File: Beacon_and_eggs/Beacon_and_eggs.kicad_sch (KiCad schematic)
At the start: 41 parts, among them J1 USB_C_Receptacle_USB2.0_16P, Q1 IRLML0030, SW1 Boot, SW2 Reset, U1 SA818V, U2 STM32F411CEUx, U3 ADXL343, U6 MCP1253-33X50I/MS, U7 MCP1253-33X50I/MS, Y1 25MHz 18pF, Y2 32.768kHz 12.5pF

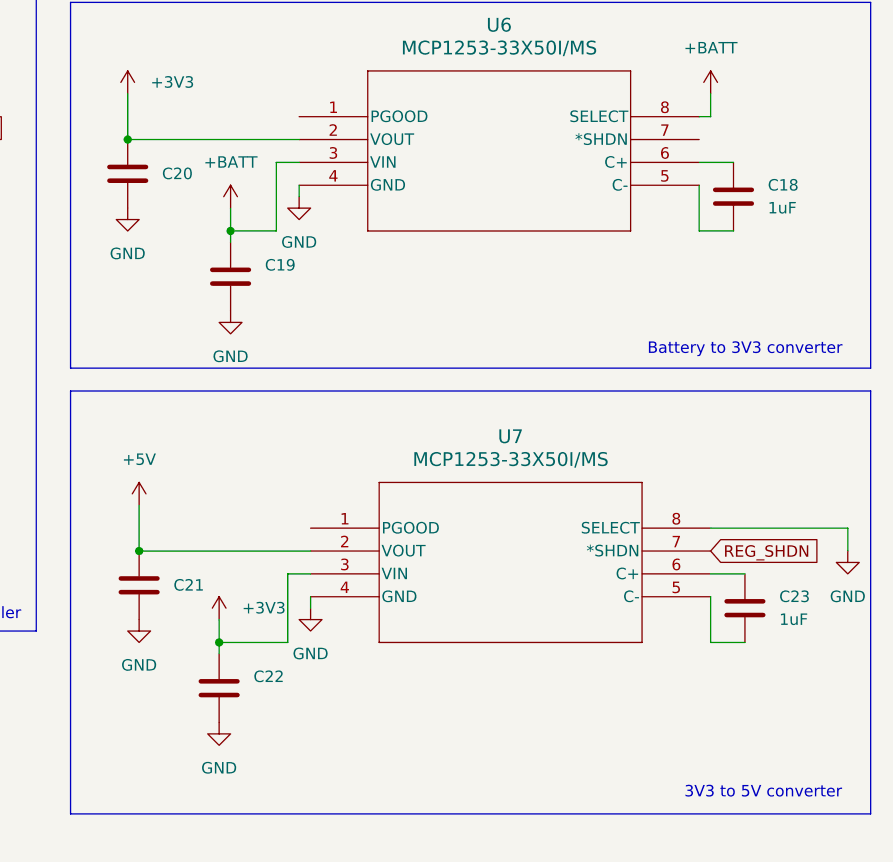
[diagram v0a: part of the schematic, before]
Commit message: Assingned most components(1206 for resistors and Capacitors)
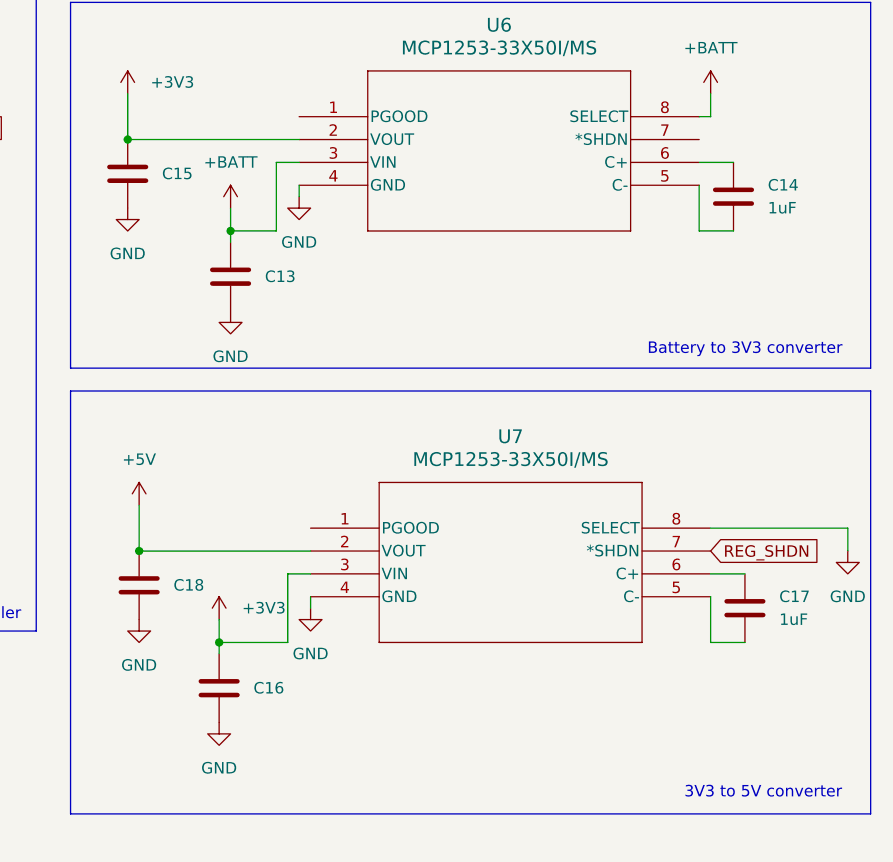
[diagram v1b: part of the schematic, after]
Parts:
- BZ1: footprint (none) -> Buzzer_Beeper:MagneticBuzzer_PUI_SMT-1028-T-2-R
- C1, C10, C11, C12, C2, C3, C4, C5, C6, C7, C8, C9: footprint (none) -> Capacitor_SMD:C_1206_3216Metric
- J1: footprint (none) -> Connector_USB:USB_C_Receptacle_HCTL_HC-TYPE-C-16P-01A
- R1, R2, R3, R4, R5, R6, R7, R8, R9: footprint (none) -> Resistor_SMD:R_1206_3216Metric
- SW1, SW2: footprint (none) -> Button_Switch_SMD:SW_SPST_PTS810
- U6, U7: footprint MSOP8_MC_MCH -> 2025_26-UVR-Beacon:MSOP8_MC_MCH
- renumbered C19 to C13, C18 to C14, C20 to C15, C22 to C16, C23 to C17, C21 to C18
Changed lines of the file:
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@@
 			)
 		)
-		(property "Footprint" ""
+		(property "Footprint" "Capacitor_SMD:C_1206_3216Metric"
 			(at 109.22 119.6848 0)
 			(effects
@@
 			)
 		)
-		(property "Footprint" "MSOP8_MC_MCH"
+		(property "Footprint" "2025_26-UVR-Beacon:MSOP8_MC_MCH"
 			(at 212.598 118.872 0)
 			(effects
@@
 			)
 		)
-		(property "Footprint" ""
+		(property "Footprint" "Resistor_SMD:R_1206_3216Metric"
 			(at 28.448 80.01 90)
 			(effects
@@
 			)
 		)
-		(property "Footprint" ""
+		(property "Footprint" "Connector_USB:USB_C_Receptacle_HCTL_HC-TYPE-C-16P-01A"
 			(at 34.29 134.62 0)
 			(effects
@@
 			)
 		)
-		(property "Footprint" ""
+		(property "Footprint" "Resistor_SMD:R_1206_3216Metric"
 			(at 31.75 41.148 90)
 			(effects
@@
 			)
 		)
-		(property "Footprint" ""
+		(property "Footprint" "Capacitor_SMD:C_1206_3216Metric"
 			(at 148.59 34.5948 0)
 			(effects
@@
 			)
 		)
-		(property "Footprint" ""
+		(property "Footprint" "Resistor_SMD:R_1206_3216Metric"
 			(at 52.07 130.048 90)
 			(effects
@@
 			)
 		)
-		(property "Footprint" ""
+		(property "Footprint" "Capacitor_SMD:C_1206_3216Metric"
 			(at 40.64 65.0748 0)
 			(effects
@@
 		(dnp no)
 		(fields_autoplaced yes)
-		(property "Reference" "C19"
-			(at 215.9 100.3299 0)
+		(property "Reference" "C13"
+			(at 215.9 101.5999 0)
 			(effects
 				(font
@@
 			(project "Beacon_and_eggs"
 				(path "/8792c0a0-2ad2-47f4-a55d-c9a646f00347"
-					(reference "C19")
+					(reference "C13")
 					(unit 1)
 				)
@@
 			)
 		)
-		(property "Footprint" ""
+		(property "Footprint" "Resistor_SMD:R_1206_3216Metric"
 			(at 24.638 80.01 90)
 			(effects
@@
 		(dnp no)
 		(fields_autoplaced yes)
-		(property "Reference" "C20"
+		(property "Reference" "C15"
 			(at 204.47 90.1699 0)
 			(effects
@@
 			(project "Beacon_and_eggs"
 				(path "/8792c0a0-2ad2-47f4-a55d-c9a646f00347"
-					(reference "C20")
+					(reference "C15")
 					(unit 1)
 				)
@@
 			)
 		)
-		(property "Footprint" ""
+		(property "Footprint" "Capacitor_SMD:C_1206_3216Metric"
 			(at 161.29 34.5948 0)
 			(effects
@@
 		(dnp no)
 		(fields_autoplaced yes)
-		(property "Reference" "C22"
-			(at 214.63 146.0499 0)
+		(property "Reference" "C16"
+			(at 214.63 147.3199 0)
 			(effects
 				(font
@@
 			(project "Beacon_and_eggs"
 				(path "/8792c0a0-2ad2-47f4-a55d-c9a646f00347"
-					(reference "C22")
+					(reference "C16")
 					(unit 1)
 				)
@@
 			)
 		)
-		(property "Footprint" ""
+		(property "Footprint" "Capacitor_SMD:C_1206_3216Metric"
 			(at 35.56 47.2948 0)
 			(effects
@@
 		(dnp no)
 		(fields_autoplaced yes)
-		(property "Reference" "C21"
+		(property "Reference" "C18"
 			(at 205.74 135.8899 0)
 			(effects
@@
 			(project "Beacon_and_eggs"
 				(path "/8792c0a0-2ad2-47f4-a55d-c9a646f00347"
-					(reference "C21")
+					(reference "C18")
 					(unit 1)
 				)
@@
 			)
 		)
-		(property "Footprint" ""
+		(property "Footprint" "Resistor_SMD:R_1206_3216Metric"
 			(at 64.008 30.48 90)
 			(effects
@@
 			)
 		)
-		(property "Footprint" ""
+		(property "Footprint" "Capacitor_SMD:C_1206_3216Metric"
 			(at 148.59 23.1648 0)
 			(effects
@@
 			)
 		)
-		(property "Footprint" ""
+		(property "Footprint" "Resistor_SMD:R_1206_3216Metric"
 			(at 108.712 170.18 90)
 			(effects
@@
 		(dnp no)
 		(fields_autoplaced yes)
-		(property "Reference" "C23"
+		(property "Reference" "C17"
 			(at 273.05 137.1599 0)
 			(effects
@@
 			(project "Beacon_and_eggs"
 				(path "/8792c0a0-2ad2-47f4-a55d-c9a646f00347"
-					(reference "C23")
+					(reference "C17")
 					(unit 1)
 				)
@@
 			)
 		)
-		(property "Footprint" ""
+		(property "Footprint" "Resistor_SMD:R_1206_3216Metric"
 			(at 52.07 124.968 90)
 			(effects
@@
 			)
 		)
-		(property "Footprint" ""
+		(property "Footprint" "Capacitor_SMD:C_1206_3216Metric"
 			(at 102.87 79.0448 0)
 			(effects
@@
 			)
 		)
-		(property "Footprint" ""
+		(property "Footprint" "Capacitor_SMD:C_1206_3216Metric"
 			(at 73.66 42.2148 0)
 			(effects
@@
 		(dnp no)
 		(fields_autoplaced yes)
-		(property "Reference" "C18"
+		(property "Reference" "C14"
 			(at 271.78 91.4399 0)
 			(effects
@@
 			(project "Beacon_and_eggs"
 				(path "/8792c0a0-2ad2-47f4-a55d-c9a646f00347"
-					(reference "C18")
+					(reference "C14")
 					(unit 1)
 				)
@@
 			)
 		)
-		(property "Footprint" ""
+		(property "Footprint" "Capacitor_SMD:C_1206_3216Metric"
 			(at 102.87 51.1048 0)
 			(effects
@@
 			)
 		)
-		(property "Footprint" ""
+		(property "Footprint" "Capacitor_SMD:C_1206_3216Metric"
 			(at 161.29 23.1648 0)
 			(effects
@@
 			)
 		)
-		(property "Footprint" ""
+		(property "Footprint" "Resistor_SMD:R_1206_3216Metric"
 			(at 104.14 168.148 90)
 			(effects
@@
 			)
 		)
-		(property "Footprint" ""
+		(property "Footprint" "Button_Switch_SMD:SW_SPST_PTS810"
 			(at 31.75 31.75 0)
 			(effects
@@
 			)
 		)
-		(property "Footprint" ""
+		(property "Footprint" "Button_Switch_SMD:SW_SPST_PTS810"
 			(at 69.85 26.67 0)
 			(effects
@@
 			)
 		)
-		(property "Footprint" ""
+		(property "Footprint" "Capacitor_SMD:C_1206_3216Metric"
 			(at 102.87 66.3448 0)
 			(effects
@@
 			)
 		)
-		(property "Footprint" ""
+		(property "Footprint" "Buzzer_Beeper:MagneticBuzzer_PUI_SMT-1028-T-2-R"
 			(at 126.365 154.94 90)
 			(effects
@@
 			)
 		)
-		(property "Footprint" ""
+		(property "Footprint" "Resistor_SMD:R_1206_3216Metric"
 			(at 46.228 30.48 90)
 			(effects
@@
 			)
 		)
-		(property "Footprint" ""
+		(property "Footprint" "Capacitor_SMD:C_1206_3216Metric"
 			(at 102.87 94.2848 0)
 			(effects
@@
 			)
 		)
-		(property "Footprint" "MSOP8_MC_MCH"
+		(property "Footprint" "2025_26-UVR-Beacon:MSOP8_MC_MCH"
 			(at 211.328 73.152 0)
 			(effects

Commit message: Revert "Assingned most components(1206 for resistors and Capacitors)"
This reverts commit 7557e7a7bd89896b141ef55f24d0591e6209fe46.
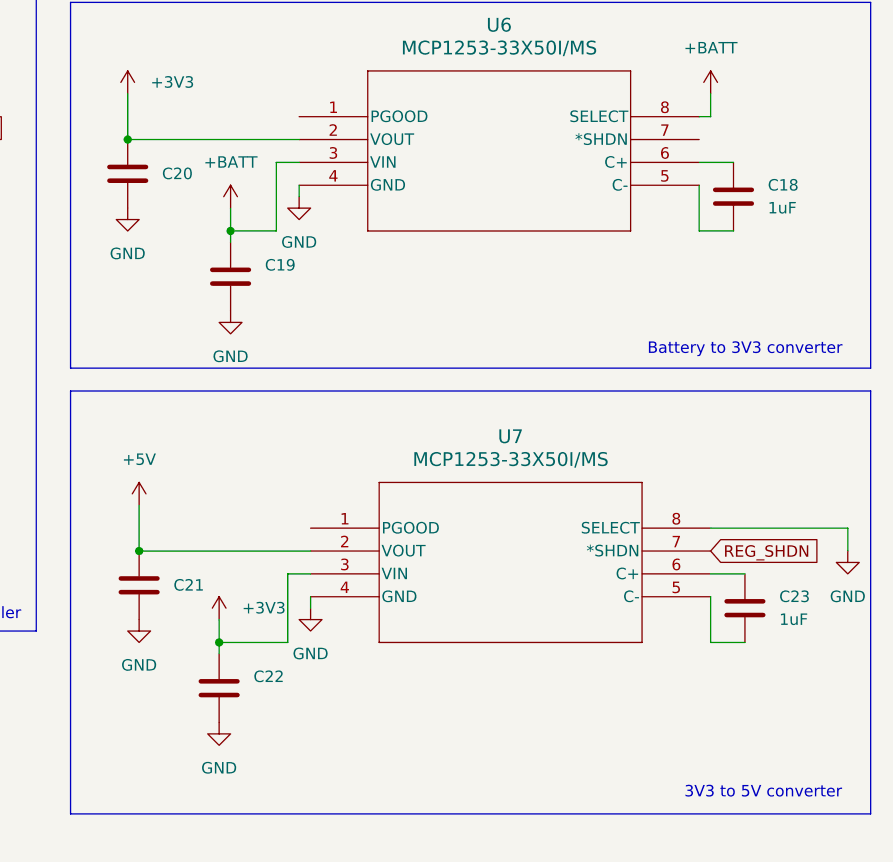
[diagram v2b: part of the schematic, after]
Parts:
- BZ1: footprint Buzzer_Beeper:MagneticBuzzer_PUI_SMT-1028-T-2-R -> (none)
- C1, C10, C11, C12, C2, C3, C4, C5, C6, C7, C8, C9: footprint Capacitor_SMD:C_1206_3216Metric -> (none)
- J1: footprint Connector_USB:USB_C_Receptacle_HCTL_HC-TYPE-C-16P-01A -> (none)
- R1, R2, R3, R4, R5, R6, R7, R8, R9: footprint Resistor_SMD:R_1206_3216Metric -> (none)
- SW1, SW2: footprint Button_Switch_SMD:SW_SPST_PTS810 -> (none)
- U6, U7: footprint 2025_26-UVR-Beacon:MSOP8_MC_MCH -> MSOP8_MC_MCH
- renumbered C14 to C18, C13 to C19, C15 to C20, C18 to C21, C16 to C22, C17 to C23
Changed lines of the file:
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@@
 			)
 		)
-		(property "Footprint" "Capacitor_SMD:C_1206_3216Metric"
+		(property "Footprint" ""
 			(at 109.22 119.6848 0)
 			(effects
@@
 			)
 		)
-		(property "Footprint" "2025_26-UVR-Beacon:MSOP8_MC_MCH"
+		(property "Footprint" "MSOP8_MC_MCH"
 			(at 212.598 118.872 0)
 			(effects
@@
 			)
 		)
-		(property "Footprint" "Resistor_SMD:R_1206_3216Metric"
+		(property "Footprint" ""
 			(at 28.448 80.01 90)
 			(effects
@@
 			)
 		)
-		(property "Footprint" "Connector_USB:USB_C_Receptacle_HCTL_HC-TYPE-C-16P-01A"
+		(property "Footprint" ""
 			(at 34.29 134.62 0)
 			(effects
@@
 			)
 		)
-		(property "Footprint" "Resistor_SMD:R_1206_3216Metric"
+		(property "Footprint" ""
 			(at 31.75 41.148 90)
 			(effects
@@
 			)
 		)
-		(property "Footprint" "Capacitor_SMD:C_1206_3216Metric"
+		(property "Footprint" ""
 			(at 148.59 34.5948 0)
 			(effects
@@
 			)
 		)
-		(property "Footprint" "Resistor_SMD:R_1206_3216Metric"
+		(property "Footprint" ""
 			(at 52.07 130.048 90)
 			(effects
@@
 			)
 		)
-		(property "Footprint" "Capacitor_SMD:C_1206_3216Metric"
+		(property "Footprint" ""
 			(at 40.64 65.0748 0)
 			(effects
@@
 		(dnp no)
 		(fields_autoplaced yes)
-		(property "Reference" "C13"
-			(at 215.9 101.5999 0)
+		(property "Reference" "C19"
+			(at 215.9 100.3299 0)
 			(effects
 				(font
@@
 			(project "Beacon_and_eggs"
 				(path "/8792c0a0-2ad2-47f4-a55d-c9a646f00347"
-					(reference "C13")
+					(reference "C19")
 					(unit 1)
 				)
@@
 			)
 		)
-		(property "Footprint" "Resistor_SMD:R_1206_3216Metric"
+		(property "Footprint" ""
 			(at 24.638 80.01 90)
 			(effects
@@
 		(dnp no)
 		(fields_autoplaced yes)
-		(property "Reference" "C15"
+		(property "Reference" "C20"
 			(at 204.47 90.1699 0)
 			(effects
@@
 			(project "Beacon_and_eggs"
 				(path "/8792c0a0-2ad2-47f4-a55d-c9a646f00347"
-					(reference "C15")
+					(reference "C20")
 					(unit 1)
 				)
@@
 			)
 		)
-		(property "Footprint" "Capacitor_SMD:C_1206_3216Metric"
+		(property "Footprint" ""
 			(at 161.29 34.5948 0)
 			(effects
@@
 		(dnp no)
 		(fields_autoplaced yes)
-		(property "Reference" "C16"
-			(at 214.63 147.3199 0)
+		(property "Reference" "C22"
+			(at 214.63 146.0499 0)
 			(effects
 				(font
@@
 			(project "Beacon_and_eggs"
 				(path "/8792c0a0-2ad2-47f4-a55d-c9a646f00347"
-					(reference "C16")
+					(reference "C22")
 					(unit 1)
 				)
@@
 			)
 		)
-		(property "Footprint" "Capacitor_SMD:C_1206_3216Metric"
+		(property "Footprint" ""
 			(at 35.56 47.2948 0)
 			(effects
@@
 		(dnp no)
 		(fields_autoplaced yes)
-		(property "Reference" "C18"
+		(property "Reference" "C21"
 			(at 205.74 135.8899 0)
 			(effects
@@
 			(project "Beacon_and_eggs"
 				(path "/8792c0a0-2ad2-47f4-a55d-c9a646f00347"
-					(reference "C18")
+					(reference "C21")
 					(unit 1)
 				)
@@
 			)
 		)
-		(property "Footprint" "Resistor_SMD:R_1206_3216Metric"
+		(property "Footprint" ""
 			(at 64.008 30.48 90)
 			(effects
@@
 			)
 		)
-		(property "Footprint" "Capacitor_SMD:C_1206_3216Metric"
+		(property "Footprint" ""
 			(at 148.59 23.1648 0)
 			(effects
@@
 			)
 		)
-		(property "Footprint" "Resistor_SMD:R_1206_3216Metric"
+		(property "Footprint" ""
 			(at 108.712 170.18 90)
 			(effects
@@
 		(dnp no)
 		(fields_autoplaced yes)
-		(property "Reference" "C17"
+		(property "Reference" "C23"
 			(at 273.05 137.1599 0)
 			(effects
@@
 			(project "Beacon_and_eggs"
 				(path "/8792c0a0-2ad2-47f4-a55d-c9a646f00347"
-					(reference "C17")
+					(reference "C23")
 					(unit 1)
 				)
@@
 			)
 		)
-		(property "Footprint" "Resistor_SMD:R_1206_3216Metric"
+		(property "Footprint" ""
 			(at 52.07 124.968 90)
 			(effects
@@
 			)
 		)
-		(property "Footprint" "Capacitor_SMD:C_1206_3216Metric"
+		(property "Footprint" ""
 			(at 102.87 79.0448 0)
 			(effects
@@
 			)
 		)
-		(property "Footprint" "Capacitor_SMD:C_1206_3216Metric"
+		(property "Footprint" ""
 			(at 73.66 42.2148 0)
 			(effects
@@
 		(dnp no)
 		(fields_autoplaced yes)
-		(property "Reference" "C14"
+		(property "Reference" "C18"
 			(at 271.78 91.4399 0)
 			(effects
@@
 			(project "Beacon_and_eggs"
 				(path "/8792c0a0-2ad2-47f4-a55d-c9a646f00347"
-					(reference "C14")
+					(reference "C18")
 					(unit 1)
 				)
@@
 			)
 		)
-		(property "Footprint" "Capacitor_SMD:C_1206_3216Metric"
+		(property "Footprint" ""
 			(at 102.87 51.1048 0)
 			(effects
@@
 			)
 		)
-		(property "Footprint" "Capacitor_SMD:C_1206_3216Metric"
+		(property "Footprint" ""
 			(at 161.29 23.1648 0)
 			(effects
@@
 			)
 		)
-		(property "Footprint" "Resistor_SMD:R_1206_3216Metric"
+		(property "Footprint" ""
 			(at 104.14 168.148 90)
 			(effects
@@
 			)
 		)
-		(property "Footprint" "Button_Switch_SMD:SW_SPST_PTS810"
+		(property "Footprint" ""
 			(at 31.75 31.75 0)
 			(effects
@@
 			)
 		)
-		(property "Footprint" "Button_Switch_SMD:SW_SPST_PTS810"
+		(property "Footprint" ""
 			(at 69.85 26.67 0)
 			(effects
@@
 			)
 		)
-		(property "Footprint" "Capacitor_SMD:C_1206_3216Metric"
+		(property "Footprint" ""
 			(at 102.87 66.3448 0)
 			(effects
@@
 			)
 		)
-		(property "Footprint" "Buzzer_Beeper:MagneticBuzzer_PUI_SMT-1028-T-2-R"
+		(property "Footprint" ""
 			(at 126.365 154.94 90)
 			(effects
@@
 			)
 		)
-		(property "Footprint" "Resistor_SMD:R_1206_3216Metric"
+		(property "Footprint" ""
 			(at 46.228 30.48 90)
 			(effects
@@
 			)
 		)
-		(property "Footprint" "Capacitor_SMD:C_1206_3216Metric"
+		(property "Footprint" ""
 			(at 102.87 94.2848 0)
 			(effects
@@
 			)
 		)
-		(property "Footprint" "2025_26-UVR-Beacon:MSOP8_MC_MCH"
+		(property "Footprint" "MSOP8_MC_MCH"
 			(at 211.328 73.152 0)
 			(effects
